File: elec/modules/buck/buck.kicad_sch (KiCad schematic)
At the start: 20 parts, among them J1 12V, J2 5V, J3 3V3, J4 GND, U2 TPS5430DDAG4, U3 TPS5430DDAG4

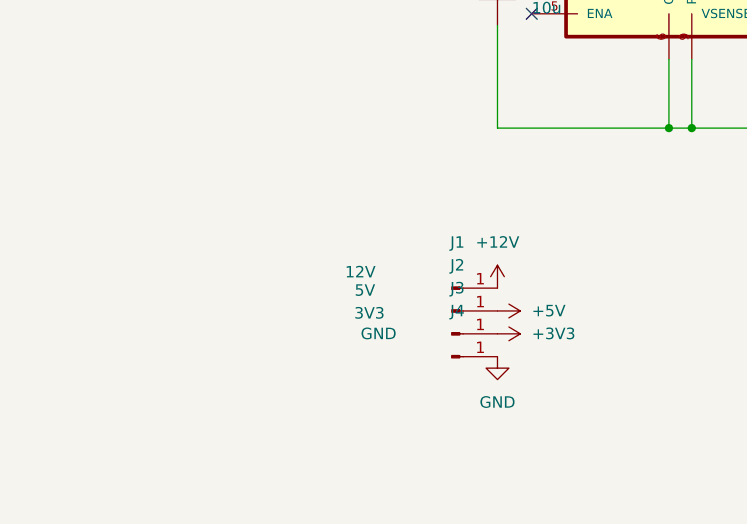
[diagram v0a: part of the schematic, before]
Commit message: sleepy but did most pcbs
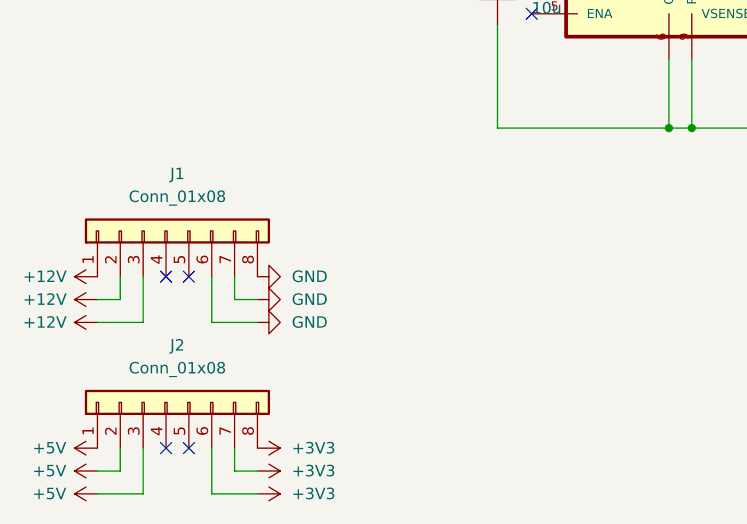
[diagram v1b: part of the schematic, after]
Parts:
- removed J1: 12V, cool custom thingy:custompadvia, symbol Connector:Conn_01x01_Pin
- removed J2: 5V, cool custom thingy:custompadvia, symbol Connector:Conn_01x01_Pin
- removed J3: 3V3, cool custom thingy:custompadvia, symbol Connector:Conn_01x01_Pin
- removed J4: GND, cool custom thingy:custompadvia, symbol Connector:Conn_01x01_Pin
- added J1, J2: Conn_01x08, Pinheaders:PinHeader_1x08_P2.54mm_Vertical, symbol Connector_Generic:Conn_01x08
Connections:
- net +12V: now also J1.1 (Pin_1), J1.2 (Pin_2), J1.3 (Pin_3)
- net +3V3: now also J2.6 (Pin_6), J2.7 (Pin_7), J2.8 (Pin_8)
- net +5V: now also J2.1 (Pin_1), J2.2 (Pin_2), J2.3 (Pin_3)
- net GND: now also J1.6 (Pin_6), J1.7 (Pin_7), J1.8 (Pin_8)
- no-connect marks 2 -> 6
